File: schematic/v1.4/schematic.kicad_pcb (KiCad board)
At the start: 4 copper layers, 85.7 x 22.9 mm, 18 parts, among them J1 USB C 2.0 8Pin, J2 PWR SW, Q1 AO3401, Q2 2N2222, U1 ESP32-C3, U2 4466, U5 WS2812B, U6 AMS1117

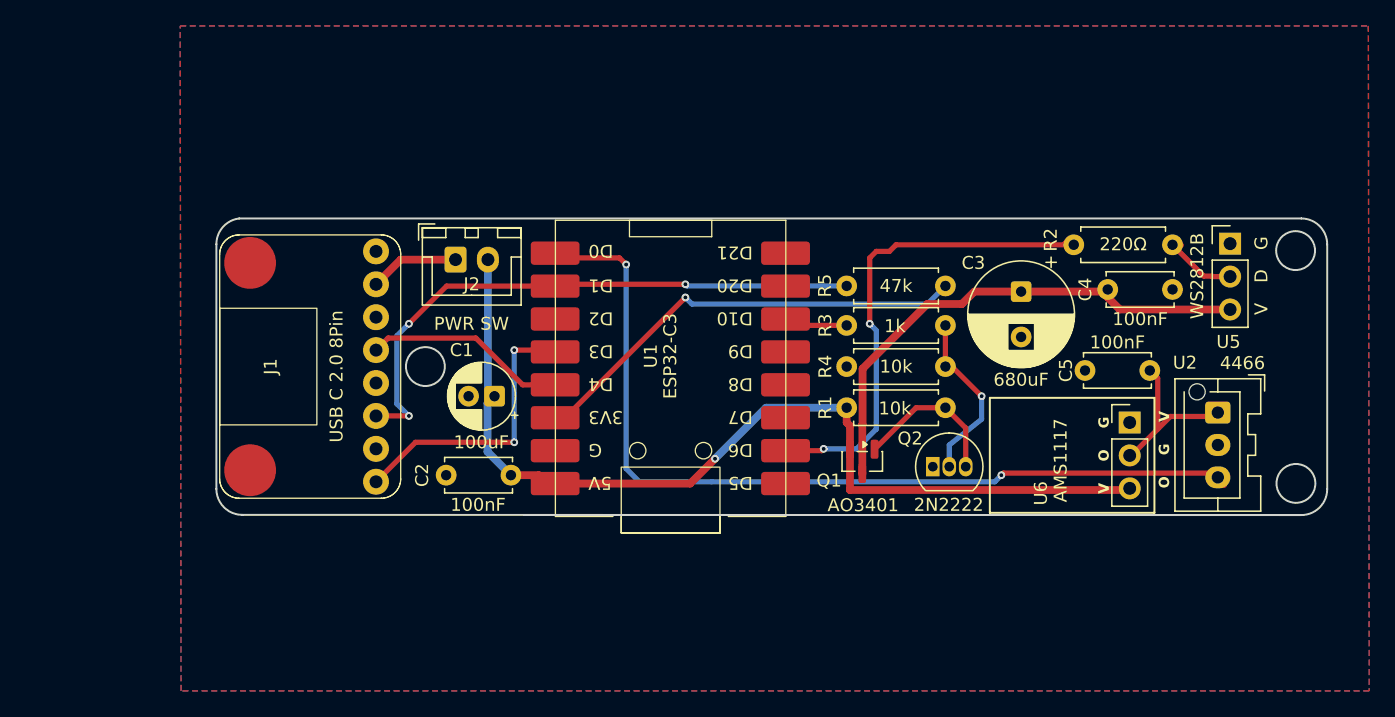
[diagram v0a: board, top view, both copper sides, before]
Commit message: Add pcb svg and updates
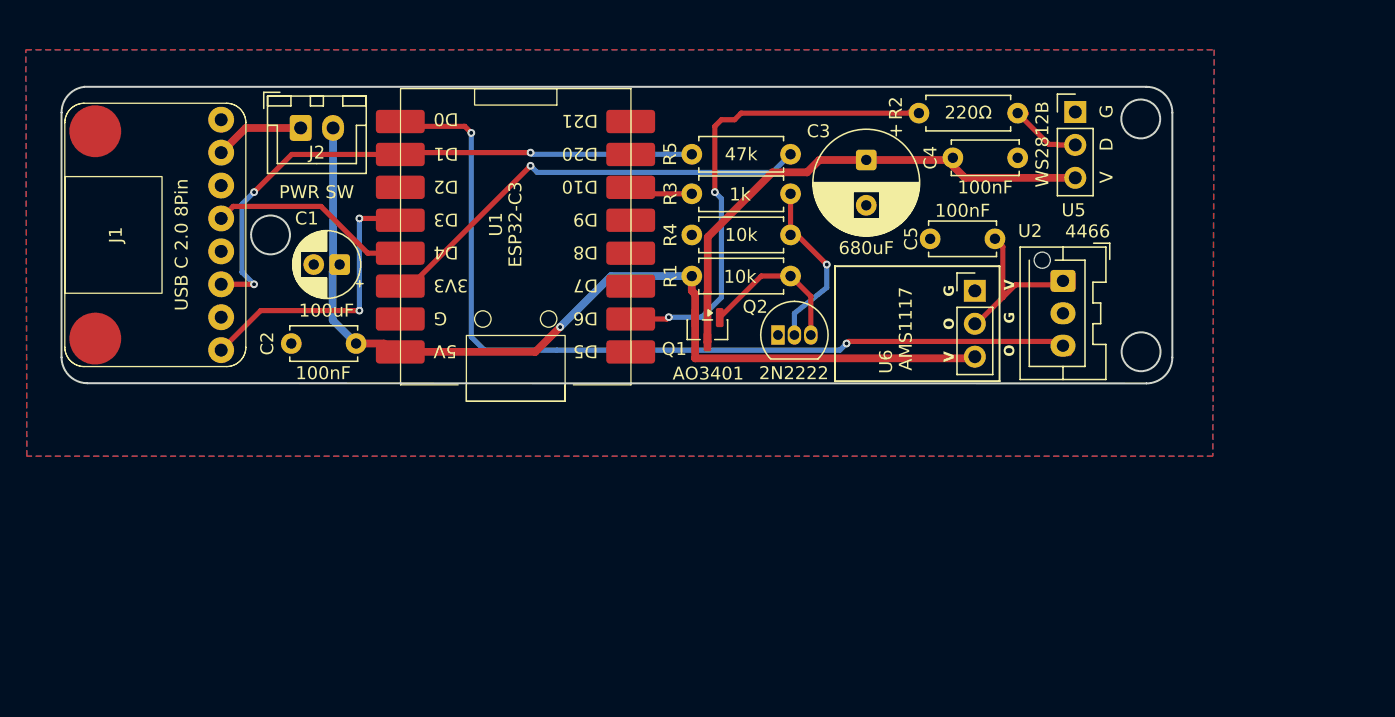
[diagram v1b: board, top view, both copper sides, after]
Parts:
- moved J1 15.7 mm to (32.1, 34.3)
- moved Q2 15.7 mm to (80.8, 42.0)
- moved R4 15.7 mm to (81.8, 34.3)
- moved U5 15.7 mm to (103.7, 24.8)
- moved U6 15.7 mm to (96.0, 38.6)
- moved C5 15.7 mm to (97.5, 34.6)
- moved J2 15.7 mm to (44.0, 26.0)
- moved Q1 15.7 mm to (75.4, 41.6)
- moved R2 15.7 mm to (91.7, 24.9)
- moved U2 15.7 mm to (102.8, 37.8)
- moved C2 15.7 mm to (48.2, 42.7)
- moved U1 15.7 mm to (60.6, 34.4)
- moved C1 15.7 mm to (47.0, 36.6)
- moved C3 15.7 mm to (87.6, 28.5)
- moved C4 15.7 mm to (99.3, 28.3)
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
